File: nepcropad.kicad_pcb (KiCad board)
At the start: 2 copper layers, 101.6 x 58.7 mm, 34 parts, among them SW1 SW_Push, U1 ATmega32U4-A, Y1 16MHz

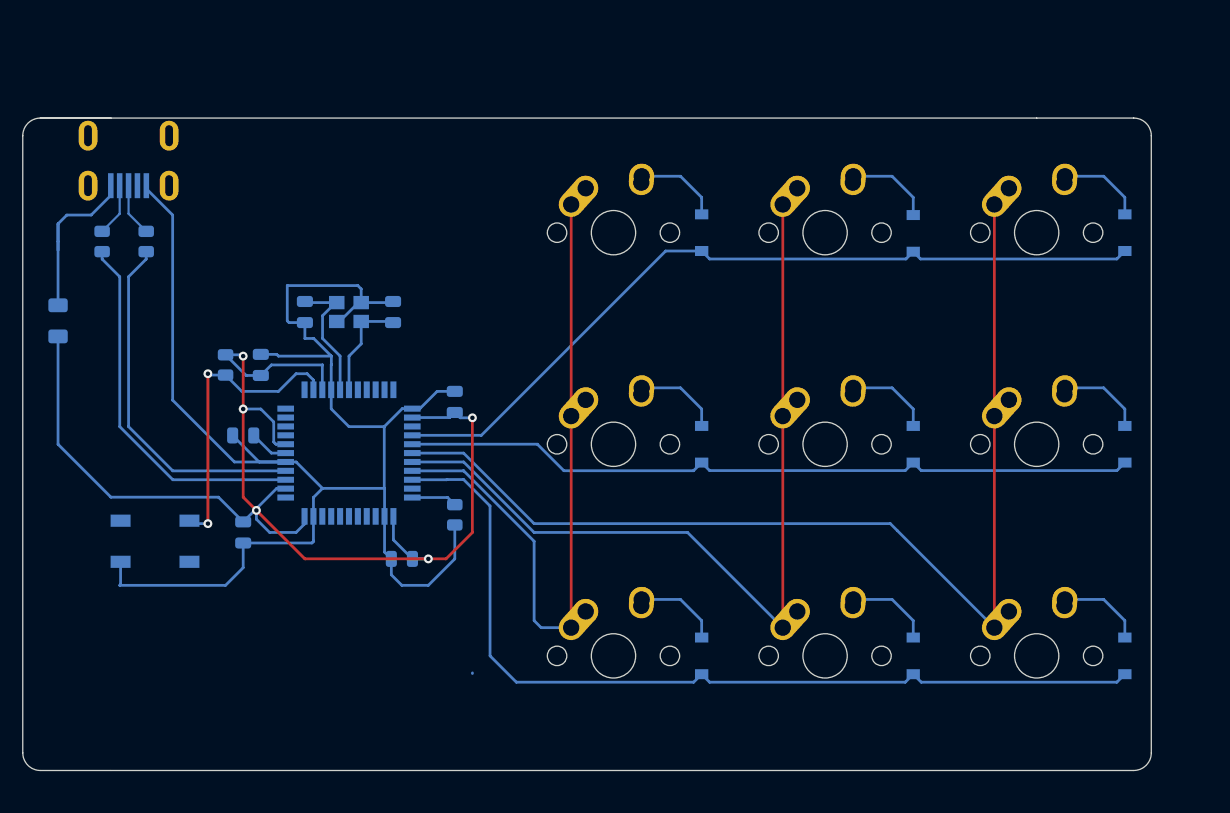
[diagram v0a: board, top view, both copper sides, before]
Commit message: minimize pcb
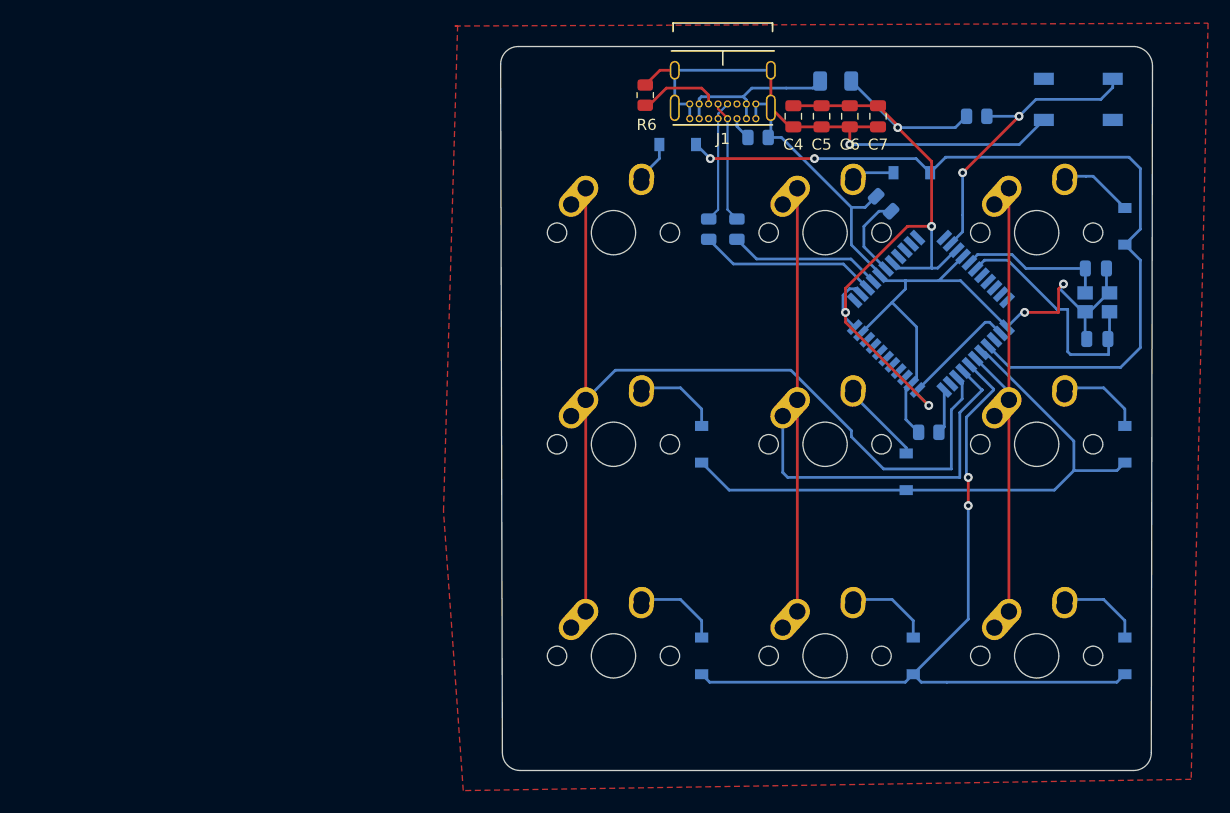
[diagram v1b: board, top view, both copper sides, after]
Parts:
- removed USB1: Molex-0548190589, random-keyboard-parts:Molex-0548190589
- added J1: USB_C_Receptacle_USB2.0, usbc:USB_C_GCT_USB4085, F.Cu at (144.8, 55.1)
- added R5: 5.1k, resistor:R_0805_2012Metric, B.Cu at (148.0, 62.9)
- added R6: 5.1k, resistor:R_0805_2012Metric, F.Cu at (137.8, 59.1)
- C4, C5, C6, C7: moved to F.Cu
- moved SW1 92.2 mm to (176.8, 59.4)
- moved F1 73.3 mm to (154.9, 57.8), turned to 0 degrees
- moved C2 71.3 mm to (178.4, 74.7), turned to 180 degrees
- moved R1 71.2 mm to (167.6, 61.0), turned to 0 degrees
- moved C7 68.3 mm to (158.8, 61.0)
- moved Y1 67.4 mm to (178.5, 77.7)
- moved C1 63.4 mm to (178.5, 81.0), turned to 0 degrees
- moved C3 61.3 mm to (159.3, 68.8), turned to 135 degrees
- moved C6 56.7 mm to (156.2, 61.0), turned to -90 degrees
- moved R3 54.6 mm to (143.5, 71.1)
- moved U1 53.9 mm to (163.5, 78.7), turned to -45 degrees
- moved R2 53.2 mm to (146.1, 71.1)
- moved C4 52.9 mm to (151.1, 61.0), turned to -90 degrees
- moved R4 43.3 mm to (163.3, 89.4), turned to 0 degrees
- moved C5 41.9 mm to (153.7, 61.0), turned to -90 degrees
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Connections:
- U1 pad 29: COL1 -> ROW2
- U1 pad 30: COL0 -> COL1
- U1 pad 31: ROW2 -> COL0
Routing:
- net COL2: track 97.0 -> 43.1 mm
- net +5V: track 119.6 -> 84.8 mm, vias 5 -> 4
- net COL0: track 62.4 -> 85.7 mm
- net Net-(R2-Pad2): track 32.2 -> 13.9 mm
- net Net-(R3-Pad2): track 33.3 -> 16.1 mm
- net GND: track 147.2 -> 132.9 mm, vias 0 -> 3
- net Net-(C1-Pad2): track 9.52 -> 22.0 mm
- net ROW1: track 66.6 -> 54.4 mm
- net ROW2: track 81.2 -> 71.2 mm, vias 0 -> 2
- net Net-(J1-PadB5): track 0.00 -> 7.41 mm
- net COL1: track 77.6 -> 70.5 mm
- net D+: track 4.77 -> 11.1 mm
- net D-: track 4.77 -> 11.1 mm
- net Net-(C3-Pad1): track 3.53 -> 7.69 mm
- net Net-(D1-Pad2): track 7.71 -> 3.96 mm
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- added copper zone on F.Cu, net GND
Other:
- board size 101.6 x 58.7 mm -> 58.7 x 65.2 mm
